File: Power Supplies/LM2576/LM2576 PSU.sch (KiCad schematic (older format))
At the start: 30 parts, among them T1 Transformer_1P_2S

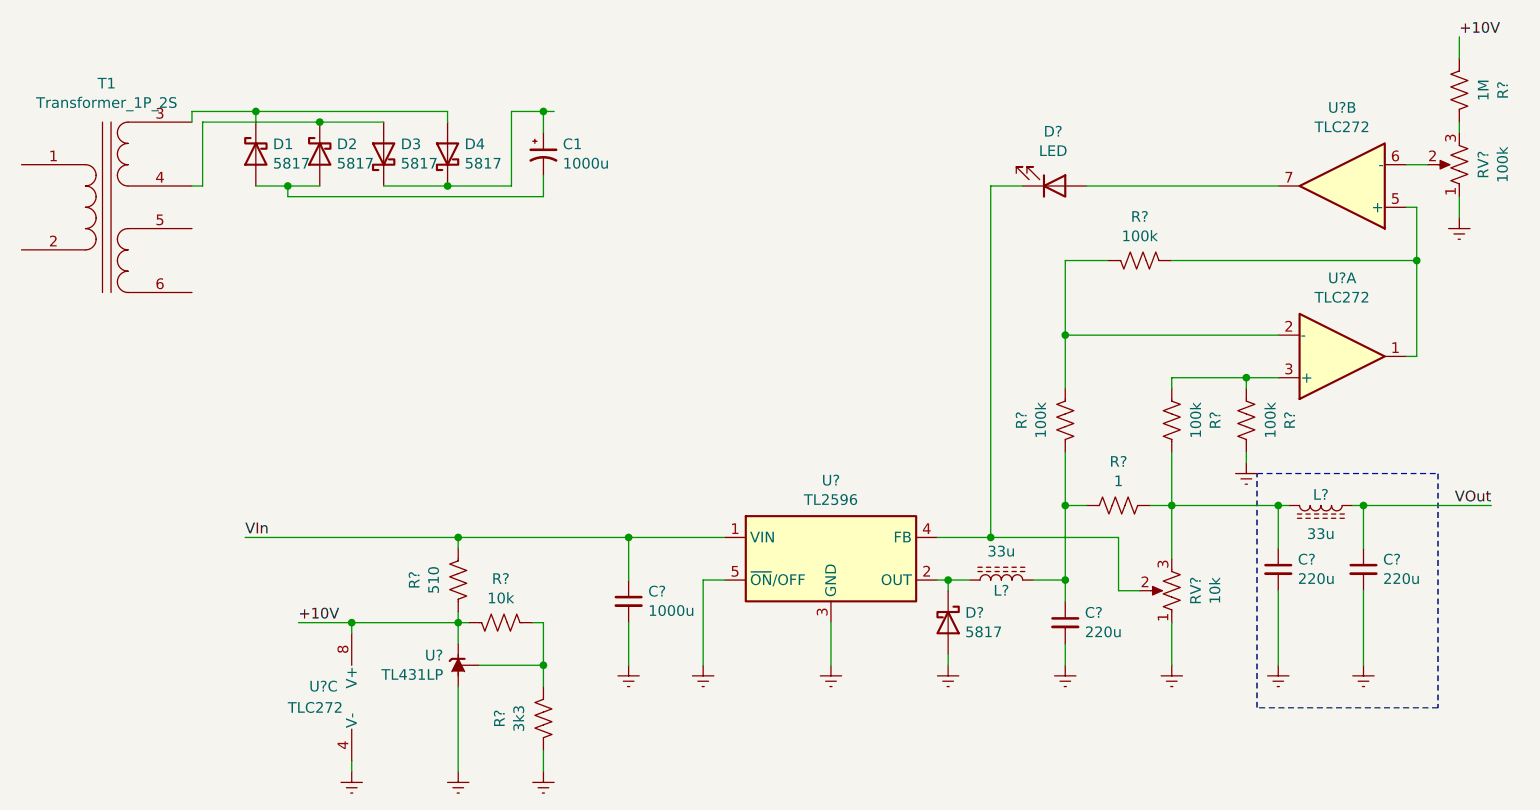
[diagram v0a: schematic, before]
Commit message: Updating latest
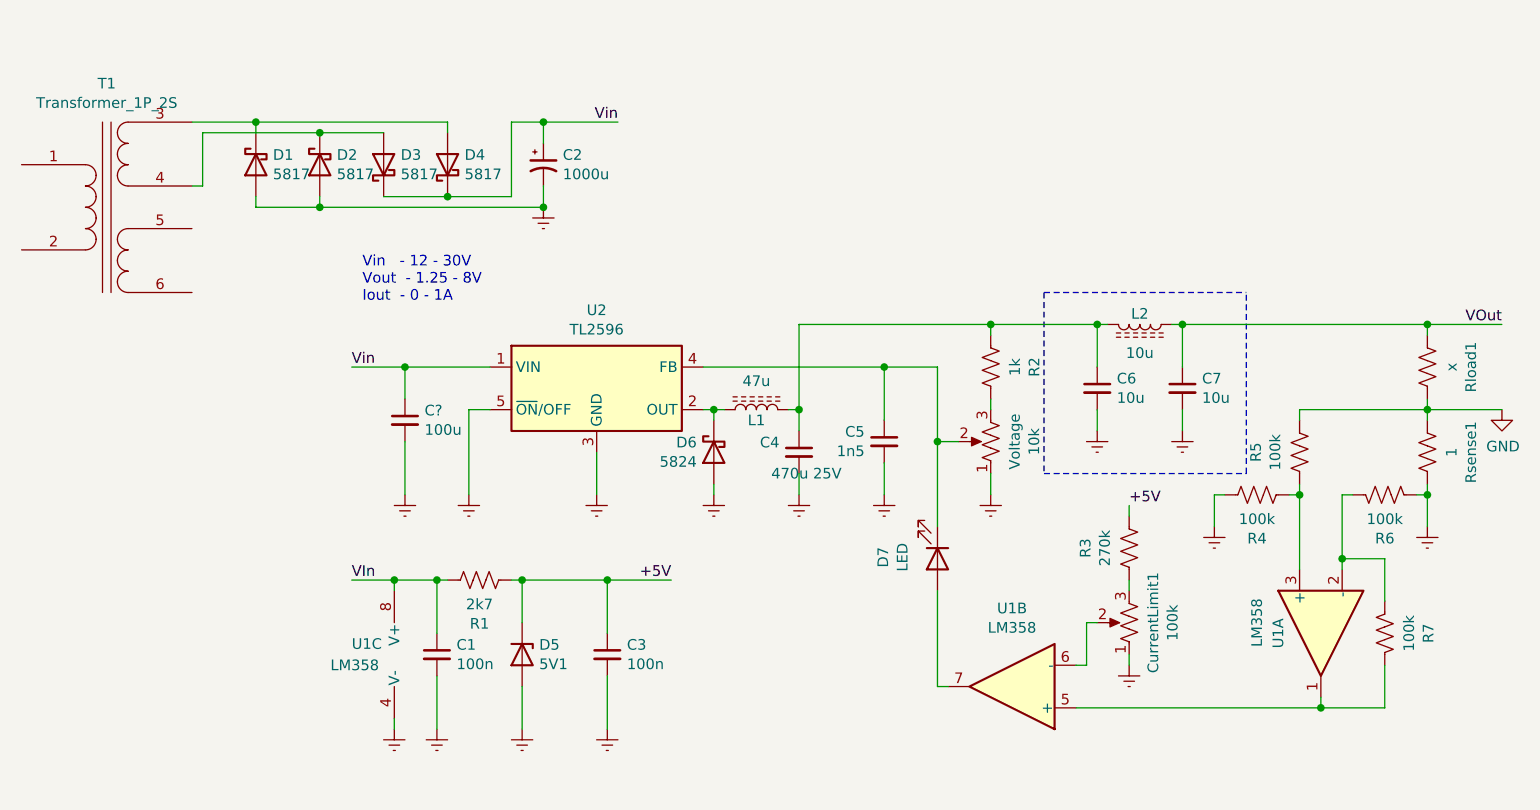
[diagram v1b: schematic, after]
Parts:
- removed C?: 1000u, symbol Device:C_Small
- removed R?: 1, symbol Device:R_US
- removed R?: 510, symbol Device:R_US
- removed R?: 10k, symbol Device:R_US
- removed R?: 3k3, symbol Device:R_US
- removed U?: TL431LP, Package_TO_SOT_THT:TO-92_Inline, symbol Reference_Voltage:TL431LP
- added C1, C3: 100n, symbol Device:C_Small
- added C5: 1n5, symbol Device:C_Small
- added C?: 100u, symbol Device:C_Small
- added D5: 5V1, symbol Device:D_Zener
- added R1: 2k7, symbol Device:R_US
- added R2: 1k, symbol Device:R_US
- added Rload1: x, symbol Device:R_US
- added Rsense1: 1, symbol Device:R_US
- C4: renamed from C?; value 220u -> 470u 25V
- C6, C7: renamed from C?; value 220u -> 10u
- D6: renamed from D?; value 5817 -> 5824
- L1: renamed from L?; value 33u -> 47u
- L2: renamed from L?; value 33u -> 10u
- R3: renamed from R?; value 1M -> 270k
- U1: renamed from U?; value TLC272 -> LM358
- gave numbers to parts that had none: 8
- renumbered C1 to C2
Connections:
- net Earth: now also C2.2, D1.2 (A), D2.2 (A), R6.2, C1.2, C3.2, C5.2, C?.2, D5.2 (A), Rsense1.2
- net VIn: now also U1.8 (V+), C1.1, R1.2; no longer U2.1 (VIN)
- net VOut: now also Rload1.1
- net Vin: now reaches C2.1, D3.1 (K), D4.1 (K)
- net Vin: now also U2.1 (VIN), C?.1
- net at D7.1 (K), U2.4 (FB), Voltage.2: now also C5.1
- net at C4.1, L1.2: now also C6.1, L2.2, R2.1; no longer R5.2
- net at R7.2, U1.2 (-): now also R6.1; no longer R5.1
- net at R4.1, U1.3 (+): now also R5.1; no longer R6.1
- net +10V renamed +5V
- net +5V: now also C3.1, D5.1 (K), R1.1; no longer U1.8 (V+)
- new net: R2.2, Voltage.3
- new net GND: R5.2, Rload1.2, Rsense1.1
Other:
- note added: "Vin - 12 - 30V\nVout - 1.25 - 8V\nIout - 0 - 1A"
- moved on the sheet: C2, C4, C6, C7, CurrentLimit1, D1, D2, D3, D4, D6, D7, L1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
